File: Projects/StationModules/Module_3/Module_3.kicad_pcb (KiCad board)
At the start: 2 copper layers, 186.7 x 90.2 mm, 34 parts, among them J1 Screw_Terminal_01x03, J2 Screw_Terminal_01x02, J4 Screw_Terminal_01x01, J5 Screw_Terminal_01x01, J6 Screw_Terminal_01x01, J7 Screw_Terminal_01x01, U1 LM2576S-5, U2 PC814

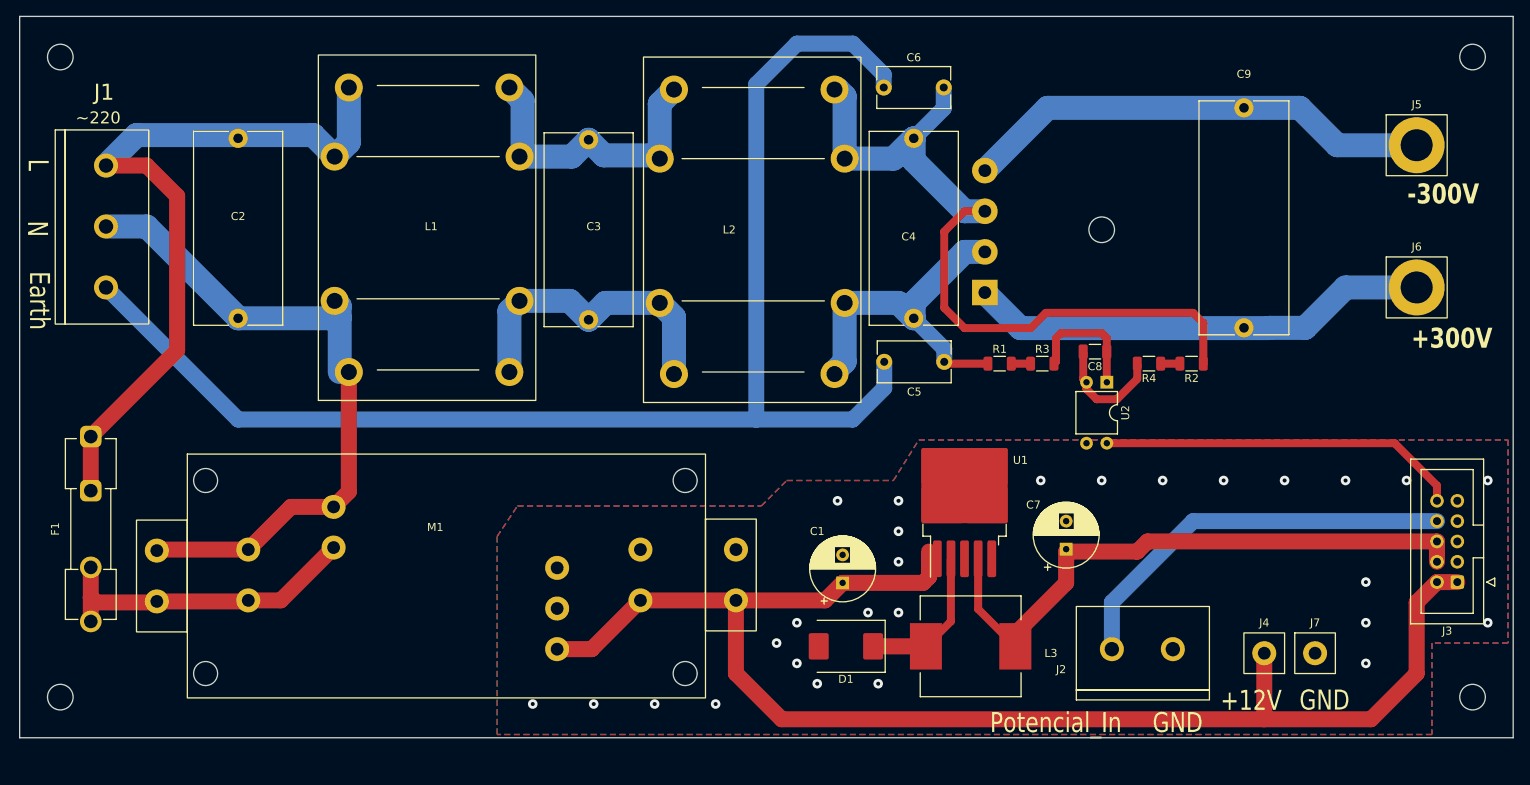
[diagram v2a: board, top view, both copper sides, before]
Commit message: change on 25_02_24
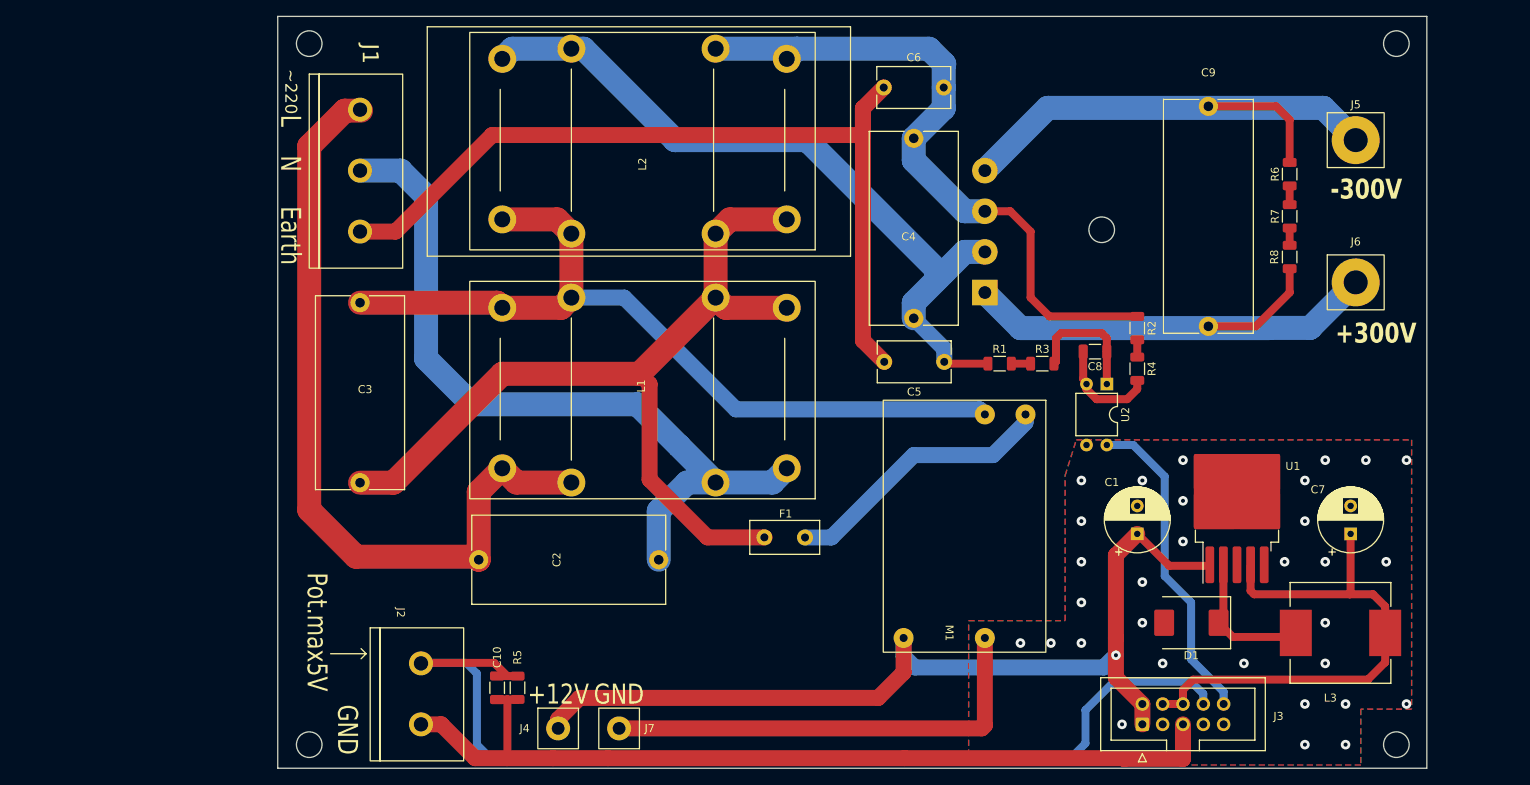
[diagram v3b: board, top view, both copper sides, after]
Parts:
- added C10: 0.1uF, Capacitor_SMD:C_1206_3216Metric, F.Cu at (107.3, 130.0)
- added R5: 1M, Resistor_SMD:R_1206_3216Metric, F.Cu at (109.9, 130.0)
- added R6: 330k, Resistor_SMD:R_1206_3216Metric, F.Cu at (206.4, 65.8)
- added R7: 330k, Resistor_SMD:R_1206_3216Metric, F.Cu at (206.4, 71.1)
- added R8: 330k, Resistor_SMD:R_1206_3216Metric, F.Cu at (206.4, 76.2)
- F1: footprint Fuse:Fuseholder_Clip-5x20mm_Keystone_3517_Inline_P23.11x6.76mm_D1.70mm_Horizontal -> Fuse:Fuse_Littelfuse_395Series
- J5, J6: footprint Z_pin:PinD4mm -> Z_pin:PinD3mm
- moved M1 107.5 mm to (175.9, 94.6), turned to -90 degrees
- moved J4 88.8 mm to (114.9, 135.1), turned to 0 degrees
- moved J7 87.5 mm to (122.6, 135.1), turned to 180 degrees
- moved J2 86.4 mm to (97.8, 127.0), turned to 0 degrees
- moved F1 85.1 mm to (140.7, 111.3), turned to 0 degrees
- moved L1 63.3 mm to (147.1, 106.4), turned to 180 degrees
- moved C2 60.6 mm to (127.5, 114.0), turned to 180 degrees
- moved L3 46.3 mm to (212.7, 123.2)
- moved D1 43.3 mm to (194.1, 121.9)
- moved J3 43.2 mm to (188.0, 134.6), turned to 90 degrees
- moved C1 37.3 mm to (187.3, 110.8)
- moved C7 35.6 mm to (214.0, 110.8)
- moved C3 35.1 mm to (90.2, 104.4)
- moved U1 34.1 mm to (199.8, 107.0)
- moved J1 32.5 mm to (90.2, 57.8)
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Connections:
- F1 pad 1: Net-(J1-Pin_1) -> Net-(C3-Pad1)
- L2 pad 3: Net-(C4-Pad2) -> Net-(C4-Pad1)
- L2 pad 4: Net-(C4-Pad1) -> Net-(C4-Pad2)
- M1 pad 1: Net-(J1-Pin_2) -> Net-(F1-Pad2)
- M1 pad 2: Net-(F1-Pad2) -> Net-(C3-Pad2)
- M1 pad 3: GND -> +12V
- M1 pad 4: +12V -> GND
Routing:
- net GND: track 0.00 -> 168.2 mm, vias 27 -> 31
- net /F_IN: track 50.7 -> 130.4 mm
- net Net-(C3-Pad1): track 38.4 -> 112.2 mm
- net Net-(J1-Pin_3): track 172.2 -> 107.7 mm
- net Net-(C3-Pad2): track 38.3 -> 102.3 mm
- net +12V: track 175.6 -> 118.2 mm, vias 0 -> 1
- net Net-(C4-Pad1): track 44.9 -> 93.6 mm
- net Net-(J1-Pin_2): track 85.2 -> 96.8 mm
- net Net-(C4-Pad2): track 96.8 -> 85.7 mm
- net +5V: track 76.8 -> 66.5 mm
- net Net-(D2--): track 59.2 -> 67.5 mm
- net Net-(D2-+): track 57.9 -> 65.5 mm
- net Net-(J1-Pin_1): track 92.4 -> 99.6 mm
- net Net-(F1-Pad2): track 40.2 -> 34.5 mm
- net /U_SET: track 45.4 -> 40.4 mm
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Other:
- board size 186.7 x 90.2 mm -> 143.6 x 94 mm
- board text added: "Pot.max5V"
- board text removed: "Potencial_In"
